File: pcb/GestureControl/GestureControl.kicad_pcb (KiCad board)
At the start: 4 copper layers, 95.3 x 87.6 mm, 102 parts, among them J1 Conn_01x04_I2I-LCD, J10 EXTERN I2C, J11 Conn_01x01, J12 Conn_01x01, J13 Conn_01x01, J14 Conn_01x01, J15 Conn_01x01, J16 Conn_01x01, J17 Conn_01x01, J18 Conn_01x01, J19 Conn_01x01, J2 BATT, J3 Conn_01x08, J4 Conn_01x06, J5 Conn_01x10, J6 Conn_01x08, J7 FTDI, J8 Serial Wire, J9 UART, SW1 SW1, SW2 SW2, SW3 BOOT, SW4 RST, U1 LD1117-3.3, U2 LD1117-5.0, U3 VL53L3CXV0DH_CENTER, U4 VL53L3CXV0DH_RIGHT, U5 VL53L3CXV0DH_LEFT, U6 STM32L151RETx, U7 STM32F401RETx, Y1 8MHz, Y2 32kHz

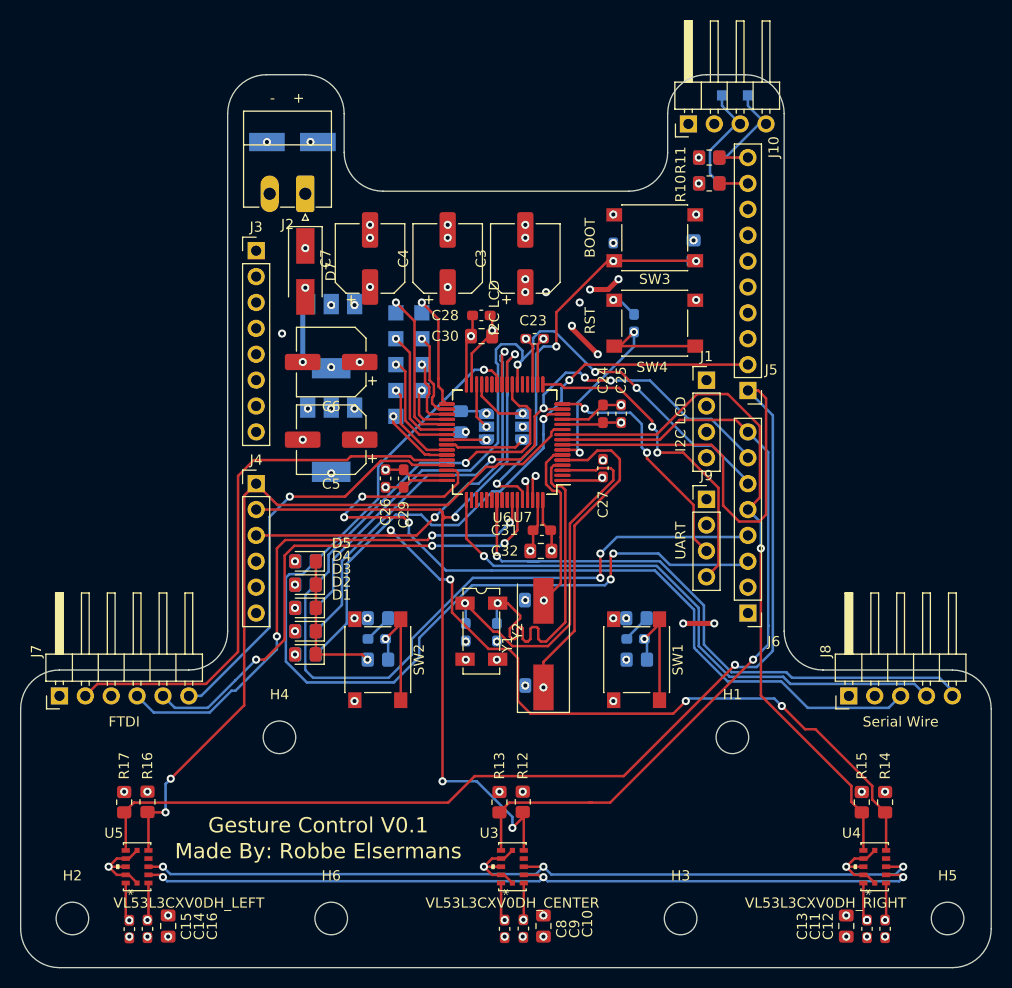
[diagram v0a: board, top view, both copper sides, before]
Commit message: eind tekenen PCB
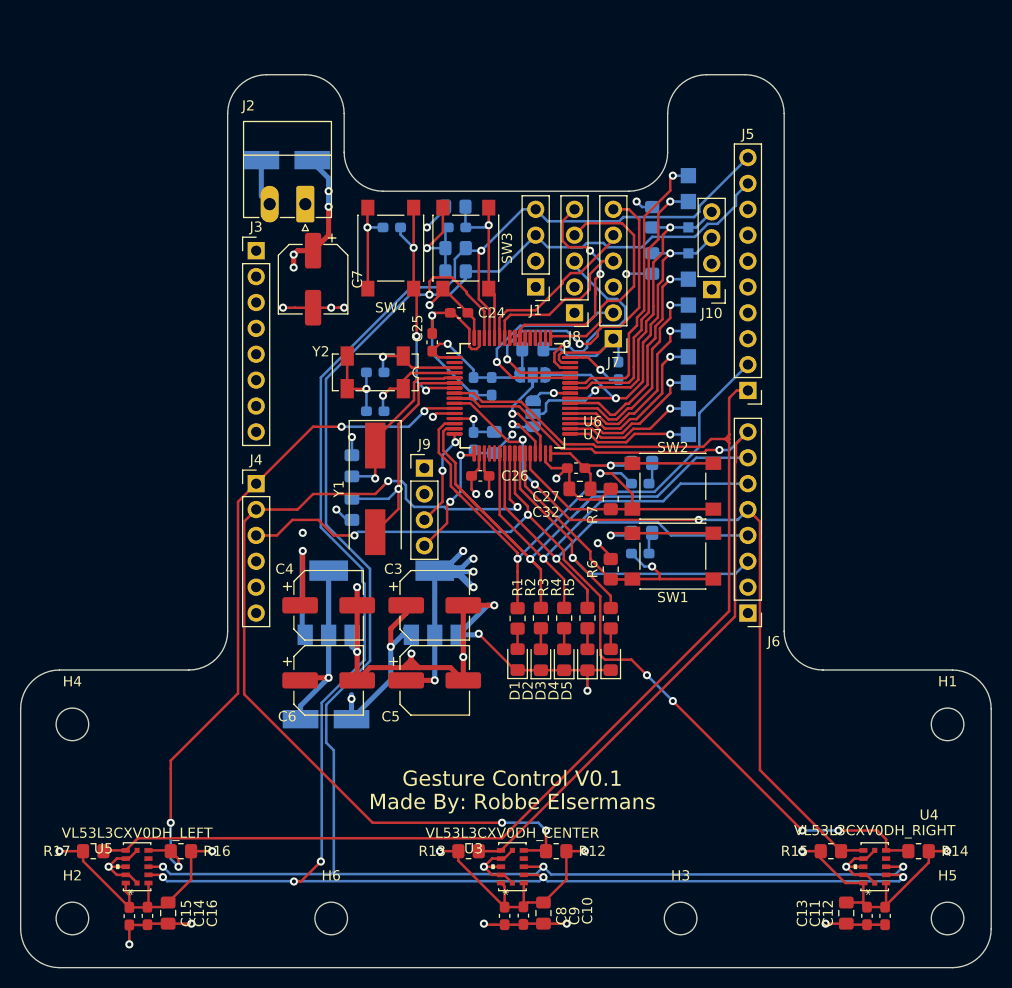
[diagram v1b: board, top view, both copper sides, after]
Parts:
- C23, C28, C29, C30, C31, D7, R10, R11: moved to B.Cu
- J10: footprint Connector_PinHeader_2.54mm:PinHeader_1x04_P2.54mm_Horizontal -> Connector_PinHeader_2.54mm:PinHeader_1x04_P2.54mm_Vertical
- J7: footprint Connector_PinHeader_2.54mm:PinHeader_1x06_P2.54mm_Horizontal -> Connector_PinHeader_2.54mm:PinHeader_1x06_P2.54mm_Vertical
- J8: footprint Connector_PinHeader_2.54mm:PinHeader_1x05_P2.54mm_Horizontal -> Connector_PinHeader_2.54mm:PinHeader_1x05_P2.54mm_Vertical
- R1, R2, R3, R4, R5, R6, R7: moved to F.Cu
- moved J7 64.7 mm to (157.0, 63.8), turned to 180 degrees
- moved J8 46.2 mm to (153.2, 61.2), turned to 180 degrees
- moved D7 44.0 mm to (128.8, 101.1), turned to 180 degrees
- moved J19 37.2 mm to (164.3, 47.8), turned to 180 degrees
- moved C4 36.0 mm to (129.0, 89.9), turned to 0 degrees
- moved C3 35.2 mm to (139.4, 89.9), turned to 0 degrees
- moved J18 34.2 mm to (164.3, 50.3), turned to 180 degrees
- moved SW2 33.6 mm to (162.8, 78.2), turned to 180 degrees
- moved D5 31.5 mm to (156.7, 95.2), turned to 90 degrees
- moved C6 31.2 mm to (129.0, 97.3), turned to 0 degrees
- moved R5 30.5 mm to (156.7, 91.2), turned to 90 degrees
- moved R9 30.1 mm to (159.8, 75.9)
- moved C2 30.0 mm to (159.6, 78.0), turned to 180 degrees
- moved J17 29.9 mm to (164.3, 57.9)
- moved J16 28.9 mm to (164.3, 60.5), turned to 180 degrees
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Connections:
- U6 pad 27: (no net) -> SW_1
- U6 pad 28: (no net) -> SW_2
- U7 pad 27: (no net) -> SW_1
- U7 pad 28: (no net) -> SW_2
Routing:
- net GND: track 89.6 -> 206.3 mm, vias 45 -> 29
- net +3V3: track 399.3 -> 506.0 mm, vias 37 -> 21
- net /STM32L151RET6TR/SWDAT: track 80.6 -> 20.3 mm, vias 3 -> 1
- net LED_5: track 94.8 -> 37.5 mm, vias 3 -> 1
- net LED_4: track 95.3 -> 39.3 mm, vias 3 -> 1
- net /STM32L151RET6TR/SW0: track 62.4 -> 23.6 mm, vias 1 -> 2
- net /STM32L151RET6TR/FTDI_TXD: track 53.1 -> 15.6 mm, vias 3 -> 0
- net /STM32L151RET6TR/SWCLK: track 57.5 -> 22.9 mm, vias 1 -> 0
- net /STM32L151RET6TR/FTDI_CTS: track 55.5 -> 22.0 mm, vias 0 -> 1
- net /STM32L151RET6TR/FTDI_RXD: track 50.3 -> 16.9 mm, vias 3 -> 0
- net LED_3: track 73.1 -> 40.9 mm, vias 3 -> 1
- net VCC: track 26.7 -> 55.5 mm, vias 4 -> 6
- net /STM32L151RET6TR/OS32_IN: track 37.0 -> 9.26 mm
- net /STM32L151RET6TR/OS32_OUT: track 35.4 -> 9.99 mm
- net GPIOI_2: track 113.2 -> 90.9 mm
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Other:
- net class PWR added: clearance 0.4, trace_width 0.25, via_dia 0.8, via_drill 0.4
- board text removed: "- +"
- board text removed: "BOOT"
- board text removed: "FTDI"
- board text removed: "I2C LCD"
- board text removed: "RST"
- board text removed: "Serial Wire"
- board text removed: "UART"
